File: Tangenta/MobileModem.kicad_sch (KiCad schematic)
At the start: 12 parts, among them J7 1-2199230-5, J8 HYC90-SIM06-180

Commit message: ...
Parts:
- C1: symbol CholaSymbolsPrjLib:C_Small -> LocalPrjLib:C_Small
- H10, H11: symbol CholaSymbolsPrjLib:MountingHole -> LocalPrjLib:MountingHole
- J7: symbol CholaSymbolsPrjLib:1-2199230-5 -> LocalPrjLib:1-2199230-5
- J8: symbol CholaSymbolsPrjLib:HYC90-SIM06-180 -> LocalPrjLib:HYC90-SIM06-180
- R2: symbol CholaSymbolsPrjLib:R_Small_US -> LocalPrjLib:R_Small_US
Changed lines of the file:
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@@
     (effects (font (size 1.27 1.27)) (justify right))
   )
-  (symbol (lib_id "CholaSymbolsPrjLib:HYC90-SIM06-180") (at 148.59 87.63 0) (unit 1)
+  (symbol (lib_id "LocalPrjLib:HYC90-SIM06-180") (at 148.59 87.63 0) (unit 1)
     (in_bom yes) (on_board yes) (dnp no) (fields_autoplaced)
     (property "Reference" "J8" (at 148.59 78.74 0)
@@
     )
   )
-  (symbol (lib_id "CholaSymbolsPrjLib:MountingHole") (at 186.055 76.2 0) (unit 1)
+  (symbol (lib_id "LocalPrjLib:MountingHole") (at 186.055 76.2 0) (unit 1)
     (in_bom yes) (on_board yes) (dnp no)
     (property "Reference" "H10" (at 188.595 76.2 0)
@@
     )
   )
-  (symbol (lib_id "CholaSymbolsPrjLib:C_Small") (at 140.97 68.58 180) (unit 1)
+  (symbol (lib_id "LocalPrjLib:C_Small") (at 140.97 68.58 180) (unit 1)
     (in_bom yes) (on_board yes) (dnp no)
     (property "Reference" "C1" (at 137.16 68.58 0)
@@
     )
   )
-  (symbol (lib_id "CholaSymbolsPrjLib:C_Small") (at 156.21 68.58 180) (unit 1)
+  (symbol (lib_id "LocalPrjLib:C_Small") (at 156.21 68.58 180) (unit 1)
     (in_bom yes) (on_board yes) (dnp no)
     (property "Reference" "C1" (at 160.02 68.58 0)
@@
     )
   )
-  (symbol (lib_id "CholaSymbolsPrjLib:R_Small_US") (at 173.99 74.93 180) (unit 1)
+  (symbol (lib_id "LocalPrjLib:R_Small_US") (at 173.99 74.93 180) (unit 1)
     (in_bom yes) (on_board yes) (dnp no)
     (property "Reference" "R2" (at 172.72 74.93 0)
@@
     )
   )
-  (symbol (lib_id "CholaSymbolsPrjLib:R_Small_US") (at 54.61 77.47 90) (unit 1)
+  (symbol (lib_id "LocalPrjLib:R_Small_US") (at 54.61 77.47 90) (unit 1)
     (in_bom yes) (on_board yes) (dnp no)
     (property "Reference" "R2" (at 53.34 76.2 90)
@@
     )
   )
-  (symbol (lib_id "CholaSymbolsPrjLib:C_Small") (at 124.46 95.25 180) (unit 1)
+  (symbol (lib_id "LocalPrjLib:C_Small") (at 124.46 95.25 180) (unit 1)
     (in_bom yes) (on_board yes) (dnp no)
     (property "Reference" "C1" (at 120.65 95.25 0)
@@
     )
   )
-  (symbol (lib_id "CholaSymbolsPrjLib:MountingHole") (at 186.055 83.82 0) (unit 1)
+  (symbol (lib_id "LocalPrjLib:MountingHole") (at 186.055 83.82 0) (unit 1)
     (in_bom yes) (on_board yes) (dnp no)
     (property "Reference" "H11" (at 188.595 83.82 0)
@@
     )
   )
-  (symbol (lib_id "CholaSymbolsPrjLib:R_Small_US") (at 92.71 57.15 270) (mirror x) (unit 1)
+  (symbol (lib_id "LocalPrjLib:R_Small_US") (at 92.71 57.15 270) (mirror x) (unit 1)
     (in_bom yes) (on_board yes) (dnp no)
     (property "Reference" "R2" (at 87.63 55.88 90)
@@
     )
   )
-  (symbol (lib_id "CholaSymbolsPrjLib:R_Small_US") (at 54.61 128.27 90) (unit 1)
+  (symbol (lib_id "LocalPrjLib:R_Small_US") (at 54.61 128.27 90) (unit 1)
     (in_bom yes) (on_board yes) (dnp no)
     (property "Reference" "R2" (at 53.34 127 90)
@@
     )
   )
-  (symbol (lib_id "CholaSymbolsPrjLib:R_Small_US") (at 124.46 104.14 180) (unit 1)
+  (symbol (lib_id "LocalPrjLib:R_Small_US") (at 124.46 104.14 180) (unit 1)
     (in_bom yes) (on_board yes) (dnp no)
     (property "Reference" "R2" (at 123.19 104.14 0)
@@
     )
   )
-  (symbol (lib_id "CholaSymbolsPrjLib:1-2199230-5") (at 73.66 44.45 90) (mirror x) (unit 1)
+  (symbol (lib_id "LocalPrjLib:1-2199230-5") (at 73.66 44.45 90) (mirror x) (unit 1)
     (in_bom yes) (on_board yes) (dnp no)
     (property "Reference" "J7" (at 66.04 46.99 90)

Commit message: Fixes, new approach.
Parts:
- C1: symbol LocalPrjLib:C_Small -> LocalSymbolsPrjLib:C_Small
- H10, H11: symbol LocalPrjLib:MountingHole -> LocalSymbolsPrjLib:MountingHole
- J7: symbol LocalPrjLib:1-2199230-5 -> LocalSymbolsPrjLib:1-2199230-5
- J8: symbol LocalPrjLib:HYC90-SIM06-180 -> LocalSymbolsPrjLib:HYC90-SIM06-180
- R2: symbol LocalPrjLib:R_Small_US -> LocalSymbolsPrjLib:R_Small_US
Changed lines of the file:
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@@
     (effects (font (size 1.27 1.27)) (justify right))
   )
-  (symbol (lib_id "LocalPrjLib:HYC90-SIM06-180") (at 148.59 87.63 0) (unit 1)
+  (symbol (lib_id "LocalSymbolsPrjLib:HYC90-SIM06-180") (at 148.59 87.63 0) (unit 1)
     (in_bom yes) (on_board yes) (dnp no) (fields_autoplaced)
     (property "Reference" "J8" (at 148.59 78.74 0)
@@
     )
   )
-  (symbol (lib_id "LocalPrjLib:MountingHole") (at 186.055 76.2 0) (unit 1)
+  (symbol (lib_id "LocalSymbolsPrjLib:MountingHole") (at 186.055 76.2 0) (unit 1)
     (in_bom yes) (on_board yes) (dnp no)
     (property "Reference" "H10" (at 188.595 76.2 0)
@@
     )
   )
-  (symbol (lib_id "LocalPrjLib:C_Small") (at 140.97 68.58 180) (unit 1)
+  (symbol (lib_id "LocalSymbolsPrjLib:C_Small") (at 140.97 68.58 180) (unit 1)
     (in_bom yes) (on_board yes) (dnp no)
     (property "Reference" "C1" (at 137.16 68.58 0)
@@
     )
   )
-  (symbol (lib_id "LocalPrjLib:C_Small") (at 156.21 68.58 180) (unit 1)
+  (symbol (lib_id "LocalSymbolsPrjLib:C_Small") (at 156.21 68.58 180) (unit 1)
     (in_bom yes) (on_board yes) (dnp no)
     (property "Reference" "C1" (at 160.02 68.58 0)
@@
     )
   )
-  (symbol (lib_id "LocalPrjLib:R_Small_US") (at 173.99 74.93 180) (unit 1)
+  (symbol (lib_id "LocalSymbolsPrjLib:R_Small_US") (at 173.99 74.93 180) (unit 1)
     (in_bom yes) (on_board yes) (dnp no)
     (property "Reference" "R2" (at 172.72 74.93 0)
@@
     )
   )
-  (symbol (lib_id "LocalPrjLib:R_Small_US") (at 54.61 77.47 90) (unit 1)
+  (symbol (lib_id "LocalSymbolsPrjLib:R_Small_US") (at 54.61 77.47 90) (unit 1)
     (in_bom yes) (on_board yes) (dnp no)
     (property "Reference" "R2" (at 53.34 76.2 90)
@@
     )
   )
-  (symbol (lib_id "LocalPrjLib:C_Small") (at 124.46 95.25 180) (unit 1)
+  (symbol (lib_id "LocalSymbolsPrjLib:C_Small") (at 124.46 95.25 180) (unit 1)
     (in_bom yes) (on_board yes) (dnp no)
     (property "Reference" "C1" (at 120.65 95.25 0)
@@
     )
   )
-  (symbol (lib_id "LocalPrjLib:MountingHole") (at 186.055 83.82 0) (unit 1)
+  (symbol (lib_id "LocalSymbolsPrjLib:MountingHole") (at 186.055 83.82 0) (unit 1)
     (in_bom yes) (on_board yes) (dnp no)
     (property "Reference" "H11" (at 188.595 83.82 0)
@@
     )
   )
-  (symbol (lib_id "LocalPrjLib:R_Small_US") (at 92.71 57.15 270) (mirror x) (unit 1)
+  (symbol (lib_id "LocalSymbolsPrjLib:R_Small_US") (at 92.71 57.15 270) (mirror x) (unit 1)
     (in_bom yes) (on_board yes) (dnp no)
     (property "Reference" "R2" (at 87.63 55.88 90)
@@
     )
   )
-  (symbol (lib_id "LocalPrjLib:R_Small_US") (at 54.61 128.27 90) (unit 1)
+  (symbol (lib_id "LocalSymbolsPrjLib:R_Small_US") (at 54.61 128.27 90) (unit 1)
     (in_bom yes) (on_board yes) (dnp no)
     (property "Reference" "R2" (at 53.34 127 90)
@@
     )
   )
-  (symbol (lib_id "LocalPrjLib:R_Small_US") (at 124.46 104.14 180) (unit 1)
+  (symbol (lib_id "LocalSymbolsPrjLib:R_Small_US") (at 124.46 104.14 180) (unit 1)
     (in_bom yes) (on_board yes) (dnp no)
     (property "Reference" "R2" (at 123.19 104.14 0)
@@
     )
   )
-  (symbol (lib_id "LocalPrjLib:1-2199230-5") (at 73.66 44.45 90) (mirror x) (unit 1)
+  (symbol (lib_id "LocalSymbolsPrjLib:1-2199230-5") (at 73.66 44.45 90) (mirror x) (unit 1)
     (in_bom yes) (on_board yes) (dnp no)
     (property "Reference" "J7" (at 66.04 46.99 90)

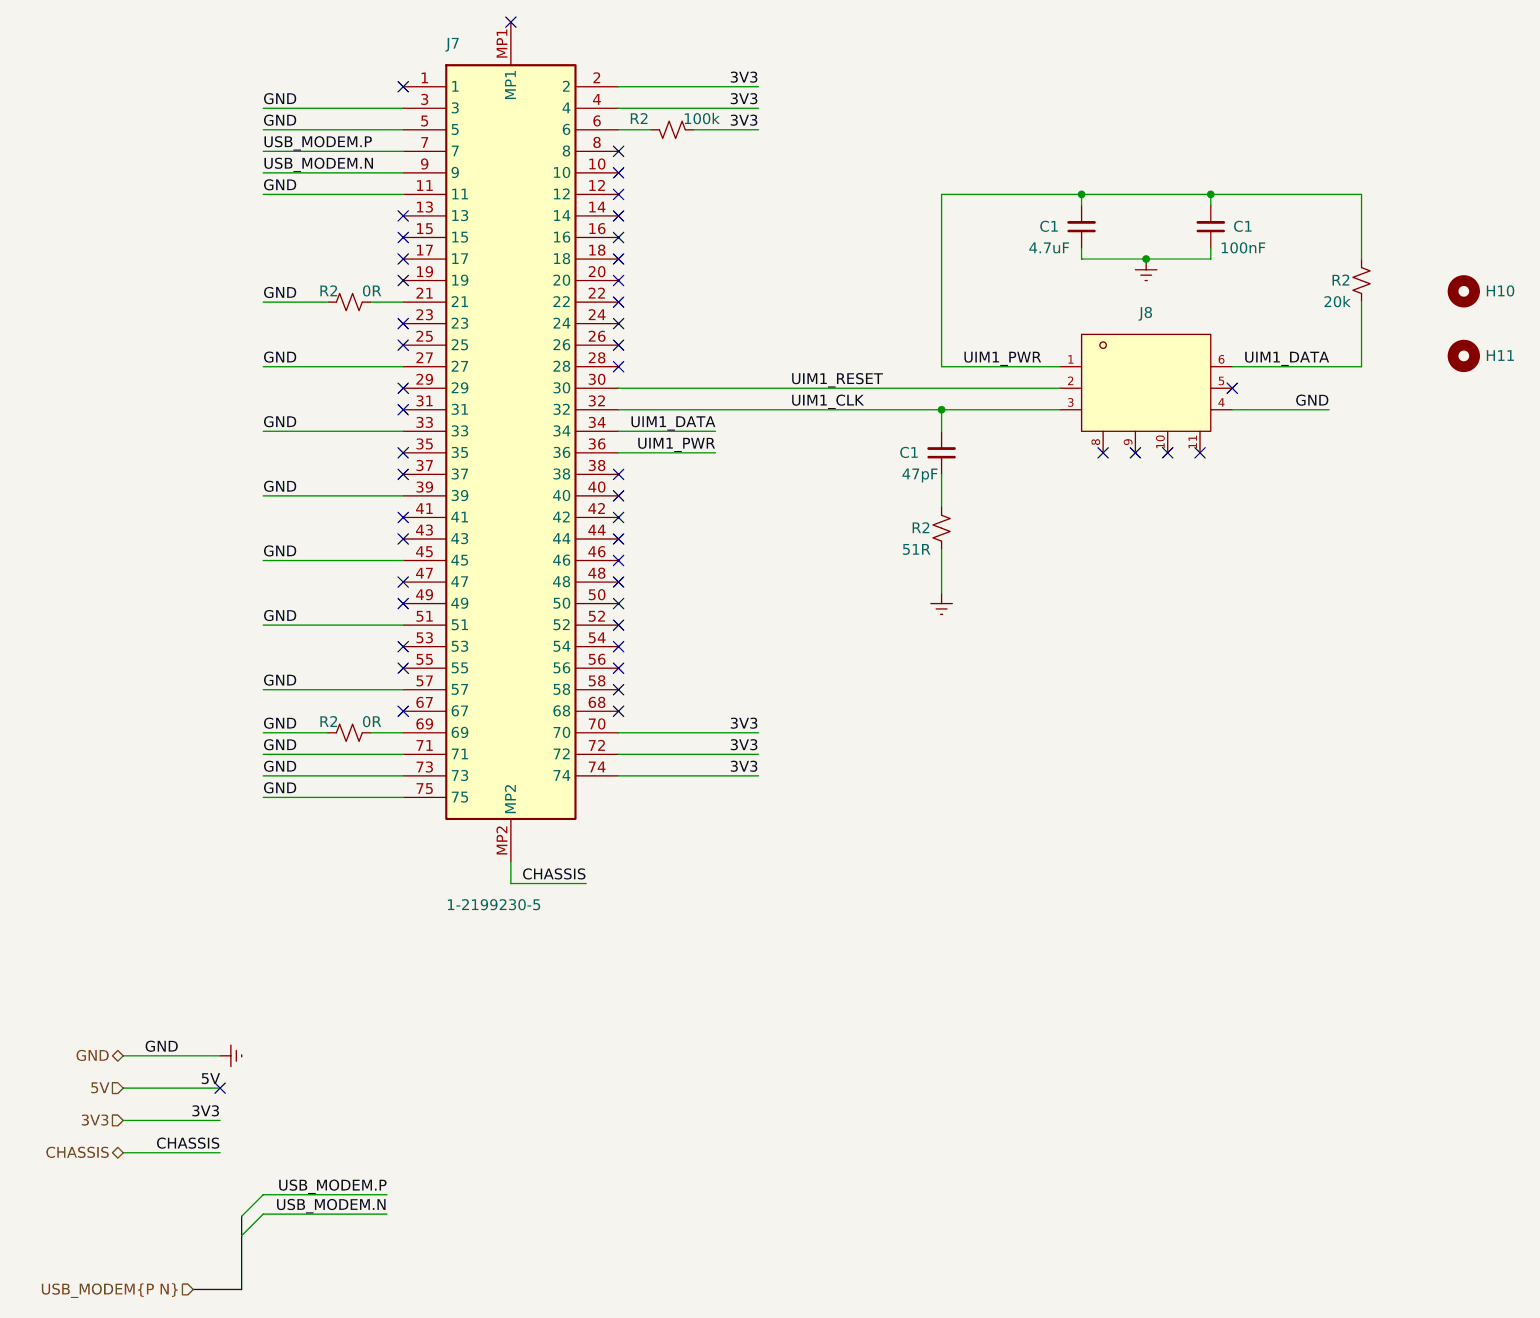
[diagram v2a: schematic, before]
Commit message: Fixes...
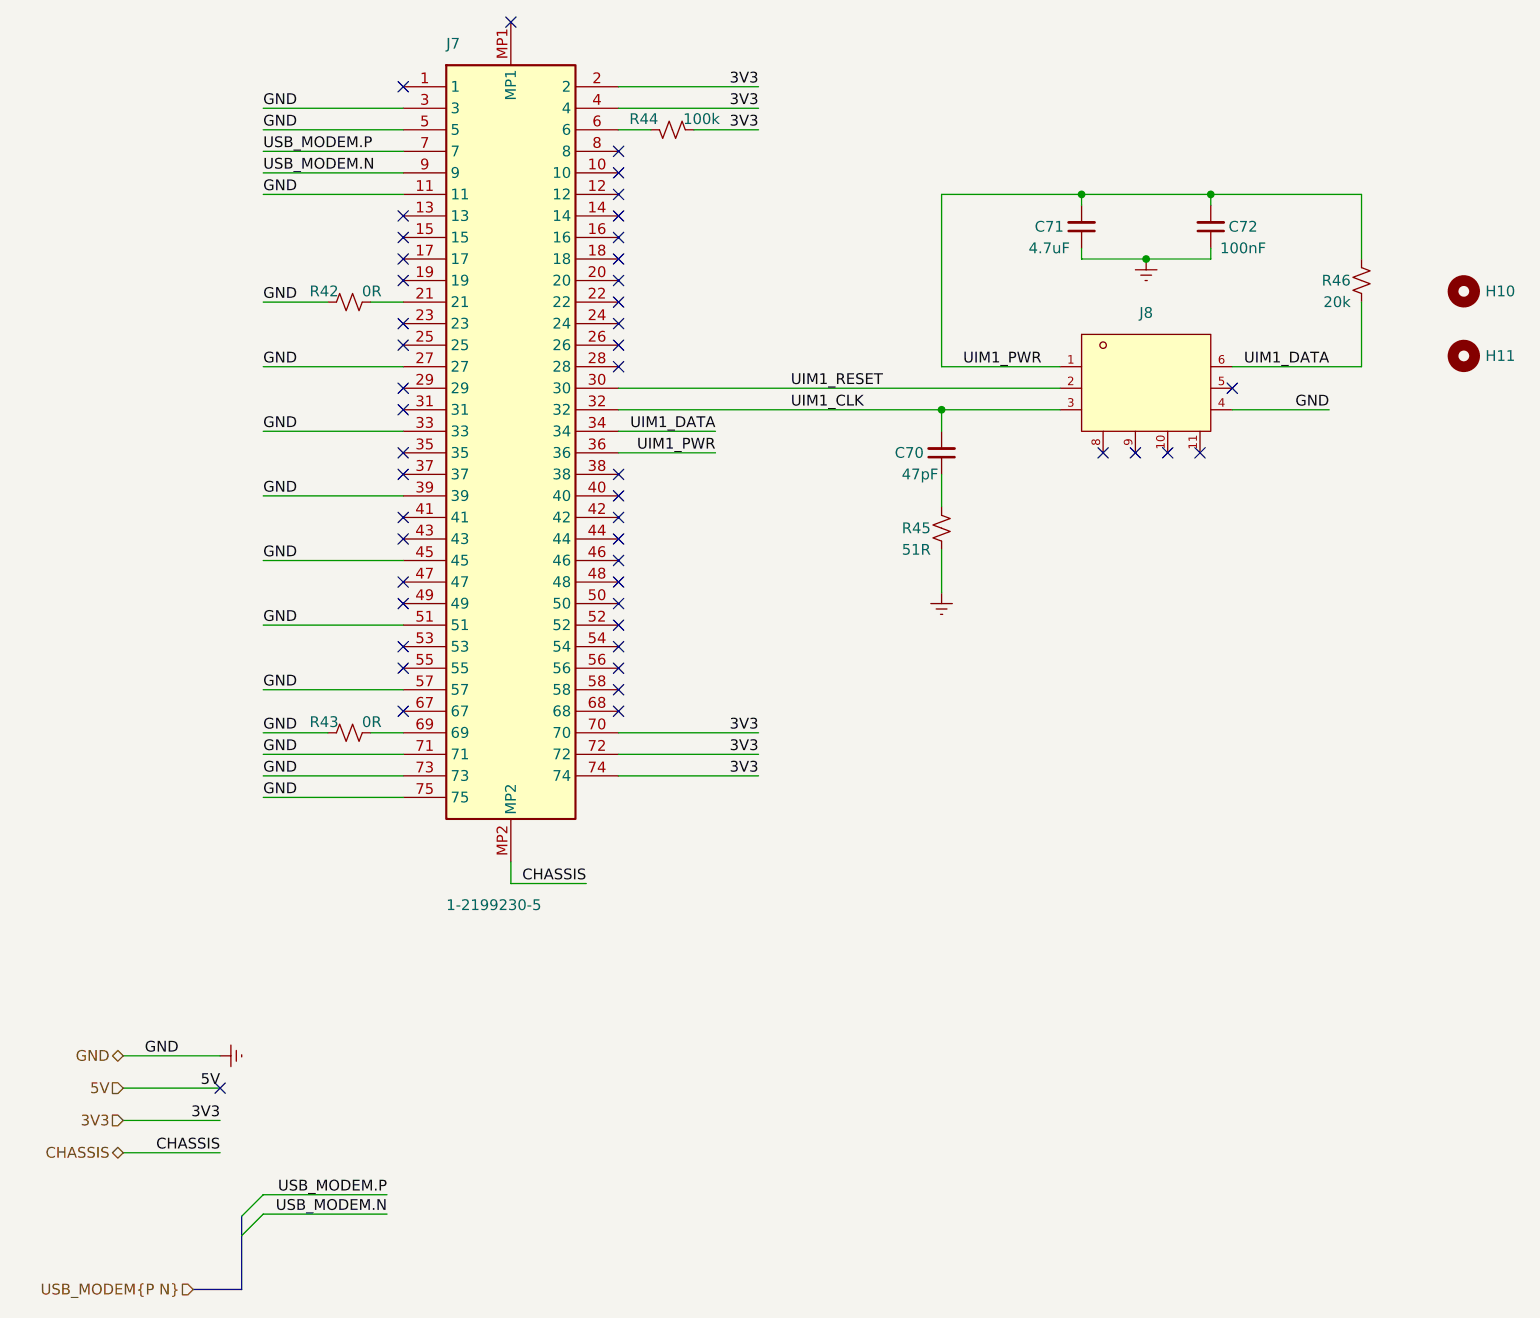
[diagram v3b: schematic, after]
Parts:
- renumbered C1 to C70, C1 to C71, C1 to C72, R2 to R42, R2 to R43, R2 to R44, R2 to R45, R2 to R46
